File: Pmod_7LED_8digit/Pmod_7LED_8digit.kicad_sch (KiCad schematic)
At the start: 12 parts, among them IC1 TM1640, J1 Pmod_Header

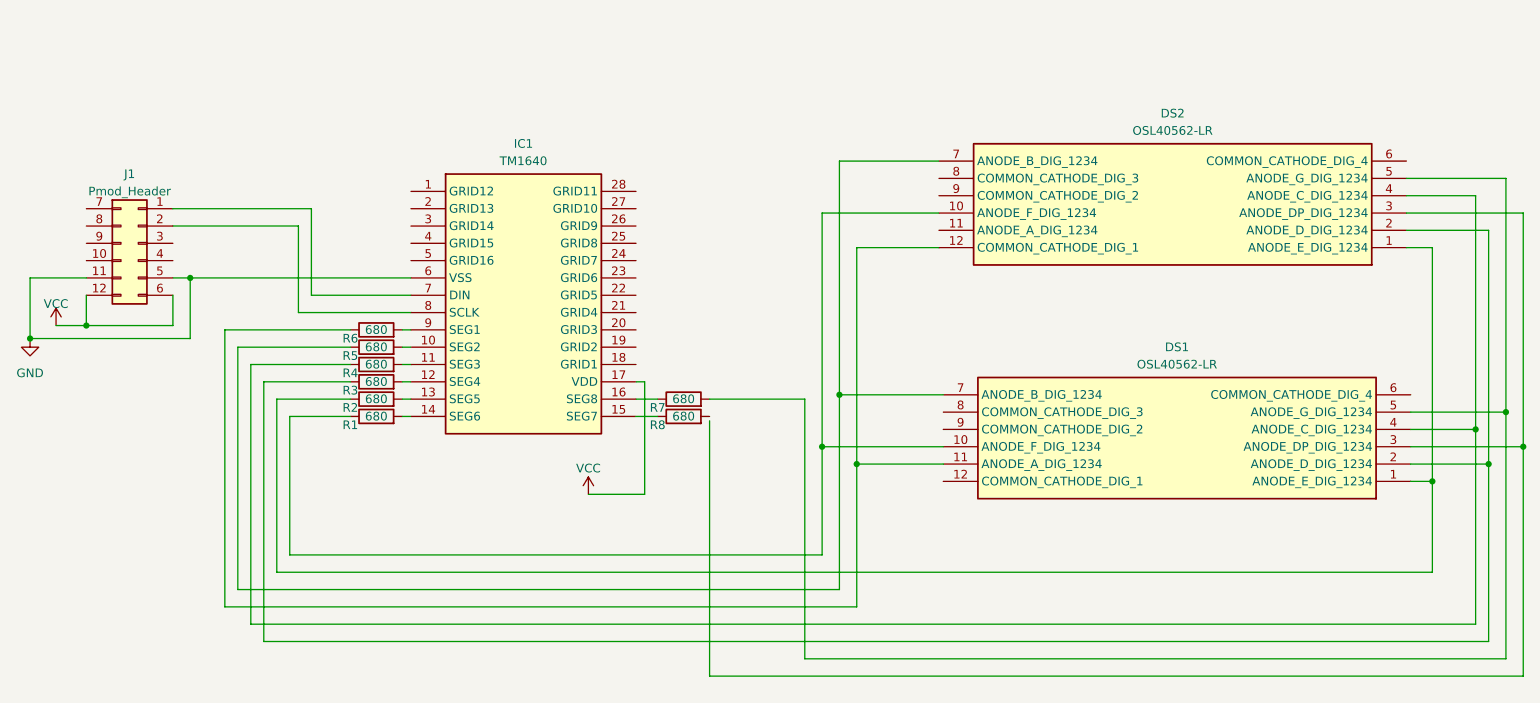
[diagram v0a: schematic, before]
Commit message: 0807
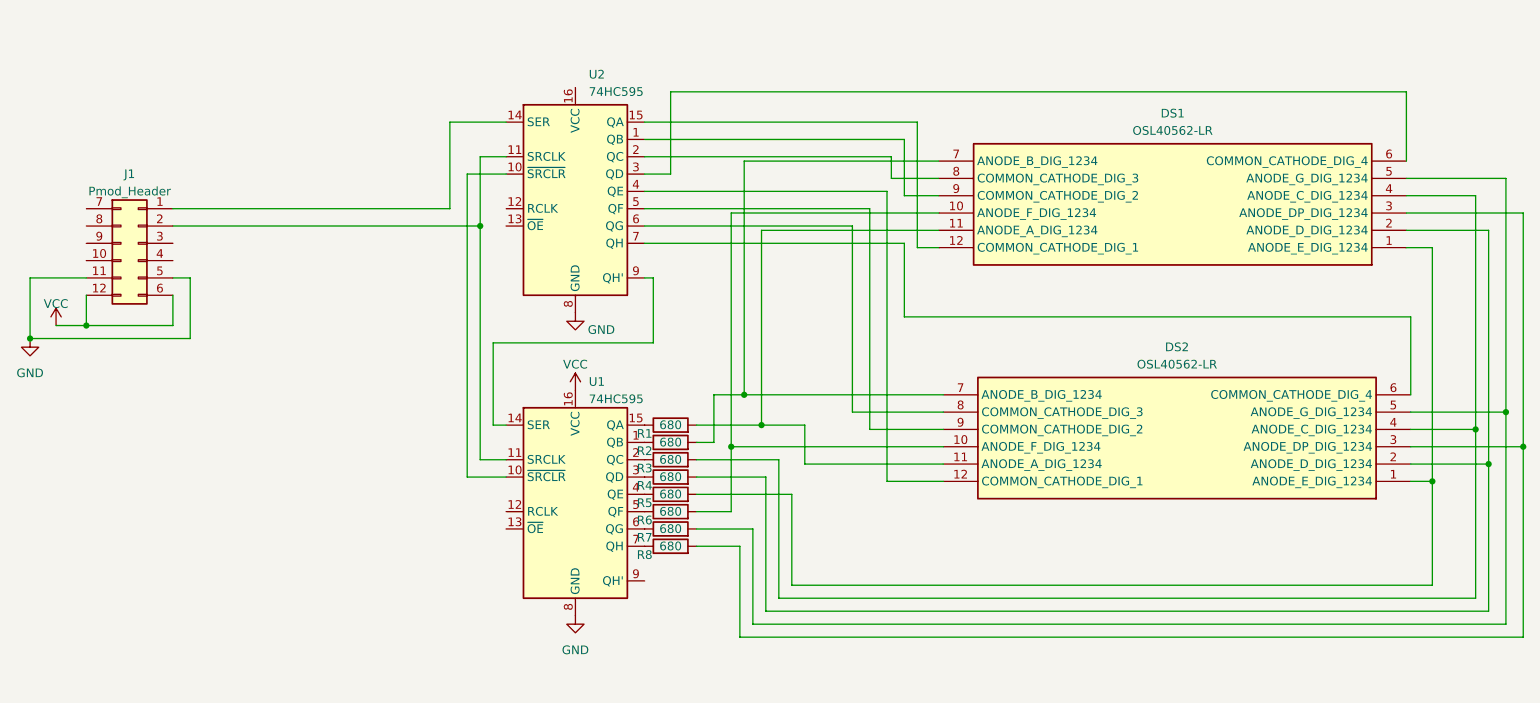
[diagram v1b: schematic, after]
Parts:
- removed IC1: TM1640, SOIC127P1020X269-28N, symbol SamacSys_Parts:TM1640
- added U1, U2: 74HC595, Package_SO:SOIC-16W_5.3x10.2mm_P1.27mm, symbol 74xx:74HC595
- renumbered DS2 to DS1, DS1 to DS2
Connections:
- net GND: now also U1.8 (GND), U2.8 (GND)
- net VCC: now also U1.16 (VCC)
- net at DS1.1 (ANODE_E_DIG_1234), DS2.1 (ANODE_E_DIG_1234): now also R5.2; no longer R2.1
- net at DS1.10 (ANODE_F_DIG_1234), DS2.10 (ANODE_F_DIG_1234): now also R6.2; no longer R1.1
- net at DS1.11 (ANODE_A_DIG_1234): now also DS2.11 (ANODE_A_DIG_1234), R1.2
- net at DS1.2 (ANODE_D_DIG_1234), DS2.2 (ANODE_D_DIG_1234): now also R4.2; no longer R3.1
- net at DS1.3 (ANODE_DP_DIG_1234), DS2.3 (ANODE_DP_DIG_1234): now also R8.2
- net at DS1.4 (ANODE_C_DIG_1234), DS2.4 (ANODE_C_DIG_1234): now also R3.2; no longer R4.1
- net at DS1.6 (COMMON_CATHODE_DIG_4): now also U2.3 (QD)
- net at DS1.7 (ANODE_B_DIG_1234), DS2.7 (ANODE_B_DIG_1234): now also R2.2; no longer R5.1
- net at DS1.8 (COMMON_CATHODE_DIG_3): now also U2.2 (QC)
- net at DS1.9 (COMMON_CATHODE_DIG_2): now also U2.1 (QB)
- net at R8.1: now also U1.7 (QH)
- net at R7.1: now also U1.6 (QG)
- net at J1.1 (Pin_1): now also U2.14 (SER)
- net at J1.2 (Pin_2): now also U1.11 (SRCLK), U2.11 (SRCLK)
- net at DS2.12 (COMMON_CATHODE_DIG_1): now also U2.4 (QE)
- net at DS2.6 (COMMON_CATHODE_DIG_4): now also U2.7 (QH)
- net at DS2.8 (COMMON_CATHODE_DIG_3): now also U2.6 (QG)
- net at DS2.9 (COMMON_CATHODE_DIG_2): now also U2.5 (QF)
- new net: DS1.12 (COMMON_CATHODE_DIG_1), U2.15 (QA)
- new net: R2.1, U1.1 (QB)
- new net: R1.1, U1.15 (QA)
- new net: U1.10 (~{SRCLR}), U2.10 (~{SRCLR})
- new net: U1.14 (SER), U2.9 (QH')
- new net: R3.1, U1.2 (QC)
- new net: R4.1, U1.3 (QD)
- new net: R5.1, U1.4 (QE)
- new net: R6.1, U1.5 (QF)
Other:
- moved on the sheet: R1, R2, R3, R4, R5, R6, R7, R8

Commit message: 0809
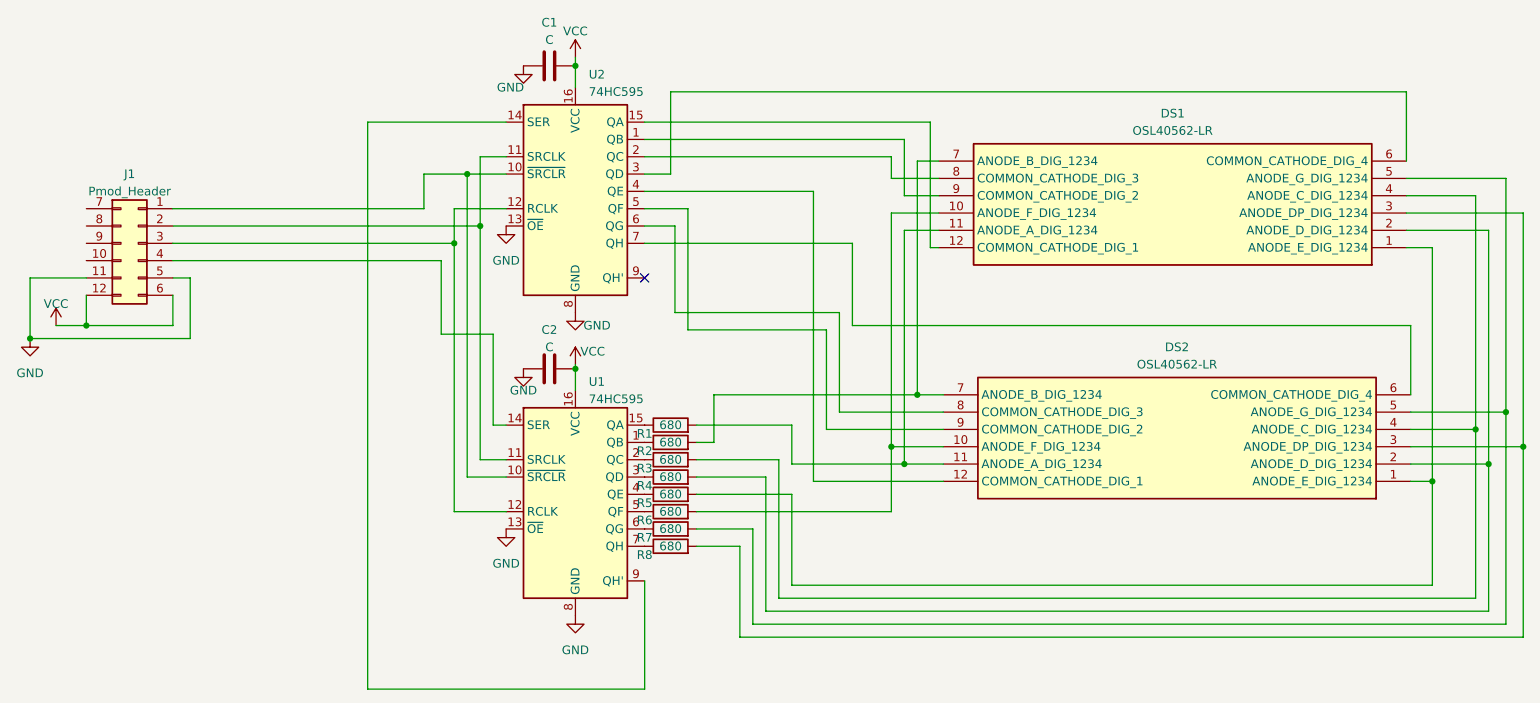
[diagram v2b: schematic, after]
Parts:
- added C1: C, Capacitor_SMD:C_0603_1608Metric_Pad1.08x0.95mm_HandSolder, symbol Device:C
- added C2: C, symbol Device:C
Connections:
- net GND: now also U1.13 (~{OE}), U2.13 (~{OE}), C1.2, C2.1
- net VCC: now also U2.16 (VCC), C1.1, C2.2
- net at U1.10 (~{SRCLR}), U2.10 (~{SRCLR}): now also J1.1 (Pin_1)
- net at U2.12 (RCLK): now also J1.3 (Pin_3), U1.12 (RCLK)
- net at U2.14 (SER): now also U1.9 (QH'); no longer J1.1 (Pin_1)
- net at U2.9 (QH'): no longer U1.14 (SER)
- net at J1.4 (Pin_4): now also U1.14 (SER)
- no-connect marks 0 -> 1

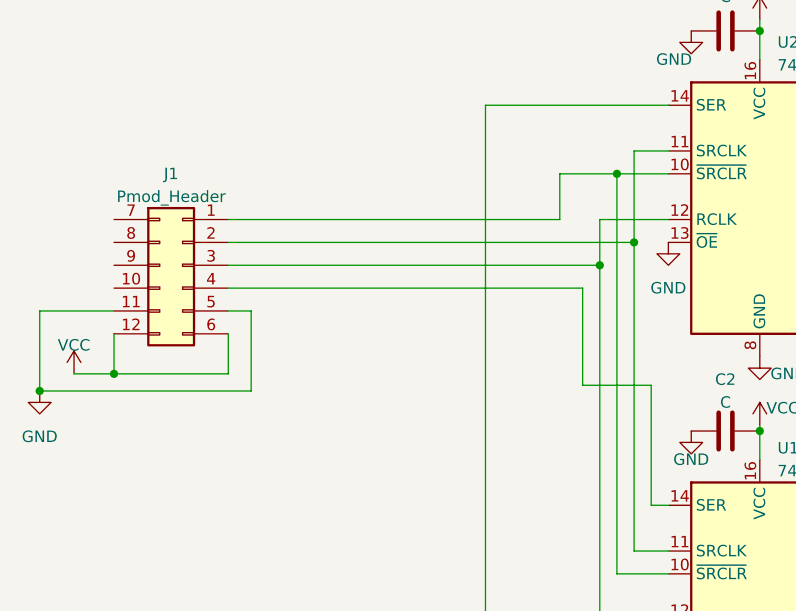
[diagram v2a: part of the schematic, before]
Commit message: 0811
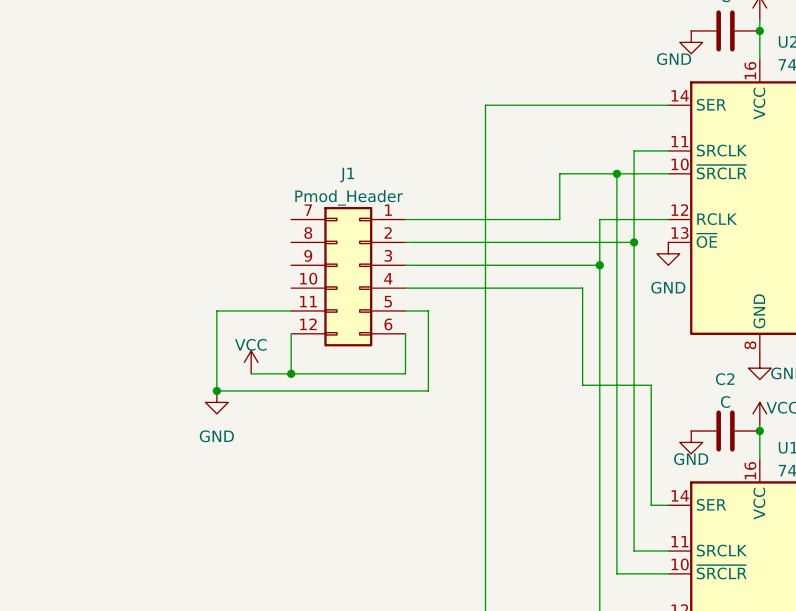
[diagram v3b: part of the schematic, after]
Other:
- moved on the sheet: J1
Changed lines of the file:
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@@
   (junction (at 111.76 67.945) (diameter 0) (color 0 0 0 0)
   )
-  (junction (at 31.75 107.95) (diameter 0) (color 0 0 0 0)
+  (junction (at 51.435 107.95) (diameter 0) (color 0 0 0 0)
   )
   (junction (at 93.98 93.98) (diameter 0) (color 0 0 0 0)
@@
   (junction (at 243.84 121.285) (diameter 0) (color 0 0 0 0)
   )
-  (junction (at 40.005 106.045) (diameter 0) (color 0 0 0 0)
+  (junction (at 59.69 106.045) (diameter 0) (color 0 0 0 0)
   )
   (junction (at 161.925 116.205) (diameter 0) (color 0 0 0 0)
@@
     (stroke (width 0) (type default))
   )
-  (wire (pts (xy 31.75 107.95) (xy 55.245 107.95))
+  (wire (pts (xy 51.435 107.95) (xy 74.93 107.95))
     (stroke (width 0) (type default))
   )
@@
     (stroke (width 0) (type default))
   )
-  (wire (pts (xy 55.245 99.06) (xy 52.705 99.06))
+  (wire (pts (xy 74.93 99.06) (xy 72.39 99.06))
     (stroke (width 0) (type default))
   )
@@
     (stroke (width 0) (type default))
   )
-  (wire (pts (xy 40.005 99.06) (xy 31.75 99.06))
+  (wire (pts (xy 59.69 99.06) (xy 51.435 99.06))
     (stroke (width 0) (type default))
   )
@@
     (stroke (width 0) (type default))
   )
-  (wire (pts (xy 52.705 88.9) (xy 89.535 88.9))
+  (wire (pts (xy 72.39 88.9) (xy 89.535 88.9))
     (stroke (width 0) (type default))
   )
@@
     (stroke (width 0) (type default))
   )
-  (wire (pts (xy 31.75 99.06) (xy 31.75 107.95))
+  (wire (pts (xy 51.435 99.06) (xy 51.435 107.95))
     (stroke (width 0) (type default))
   )
@@
     (stroke (width 0) (type default))
   )
-  (wire (pts (xy 52.705 101.6) (xy 52.705 106.045))
+  (wire (pts (xy 72.39 101.6) (xy 72.39 106.045))
     (stroke (width 0) (type default))
   )
@@
     (stroke (width 0) (type default))
   )
-  (wire (pts (xy 52.705 91.44) (xy 97.79 91.44))
+  (wire (pts (xy 72.39 91.44) (xy 97.79 91.44))
     (stroke (width 0) (type default))
   )
@@
     (stroke (width 0) (type default))
   )
-  (wire (pts (xy 92.075 96.52) (xy 52.705 96.52))
+  (wire (pts (xy 92.075 96.52) (xy 72.39 96.52))
     (stroke (width 0) (type default))
   )
@@
     (stroke (width 0) (type default))
   )
-  (wire (pts (xy 52.705 106.045) (xy 40.005 106.045))
+  (wire (pts (xy 72.39 106.045) (xy 59.69 106.045))
     (stroke (width 0) (type default))
   )
@@
     (stroke (width 0) (type default))
   )
-  (wire (pts (xy 35.56 106.045) (xy 40.005 106.045))
-    (stroke (width 0) (type default))
-  )
-  (wire (pts (xy 52.705 93.98) (xy 93.98 93.98))
+  (wire (pts (xy 55.245 106.045) (xy 59.69 106.045))
+    (stroke (width 0) (type default))
+  )
+  (wire (pts (xy 72.39 93.98) (xy 93.98 93.98))
     (stroke (width 0) (type default))
   )
@@
     (stroke (width 0) (type default))
   )
-  (wire (pts (xy 40.005 106.045) (xy 40.005 101.6))
+  (wire (pts (xy 59.69 106.045) (xy 59.69 101.6))
     (stroke (width 0) (type default))
   )
@@
     (stroke (width 0) (type default))
   )
-  (wire (pts (xy 55.245 99.06) (xy 55.245 107.95))
+  (wire (pts (xy 74.93 99.06) (xy 74.93 107.95))
     (stroke (width 0) (type default))
   )
@@
     )
   )
-  (symbol (lib_id "power:GND") (at 31.75 107.95 0) (unit 1)
+  (symbol (lib_id "power:GND") (at 51.435 107.95 0) (unit 1)
     (in_bom yes) (on_board yes) (dnp no) (fields_autoplaced)
-    (property "Reference" "#PWR03" (at 31.75 114.3 0)
-      (effects (font (size 1.27 1.27)) hide)
-    )
-    (property "Value" "GND" (at 31.75 113.03 0)
-      (effects (font (size 1.27 1.27)))
-    )
-    (property "Footprint" "" (at 31.75 107.95 0)
-      (effects (font (size 1.27 1.27)) hide)
-    )
-    (property "Datasheet" "" (at 31.75 107.95 0)
+    (property "Reference" "#PWR03" (at 51.435 114.3 0)
+      (effects (font (size 1.27 1.27)) hide)
+    )
+    (property "Value" "GND" (at 51.435 113.03 0)
+      (effects (font (size 1.27 1.27)))
+    )
+    (property "Footprint" "" (at 51.435 107.95 0)
+      (effects (font (size 1.27 1.27)) hide)
+    )
+    (property "Datasheet" "" (at 51.435 107.95 0)
       (effects (font (size 1.27 1.27)) hide)
     )
@@
     )
   )
-  (symbol (lib_id "power:VCC") (at 35.56 106.045 0) (unit 1)
+  (symbol (lib_id "power:VCC") (at 55.245 106.045 0) (unit 1)
     (in_bom yes) (on_board yes) (dnp no) (fields_autoplaced)
-    (property "Reference" "#PWR02" (at 35.56 109.855 0)
-      (effects (font (size 1.27 1.27)) hide)
-    )
-    (property "Value" "VCC" (at 35.56 102.87 0)
-      (effects (font (size 1.27 1.27)))
-    )
-    (property "Footprint" "" (at 35.56 106.045 0)
-      (effects (font (size 1.27 1.27)) hide)
-    )
-    (property "Datasheet" "" (at 35.56 106.045 0)
+    (property "Reference" "#PWR02" (at 55.245 109.855 0)
+      (effects (font (size 1.27 1.27)) hide)
+    )
+    (property "Value" "VCC" (at 55.245 102.87 0)
+      (effects (font (size 1.27 1.27)))
+    )
+    (property "Footprint" "" (at 55.245 106.045 0)
+      (effects (font (size 1.27 1.27)) hide)
+    )
+    (property "Datasheet" "" (at 55.245 106.045 0)
       (effects (font (size 1.27 1.27)) hide)
     )
@@
     )
   )
-  (symbol (lib_id "MyLibrary:Pmod_Header") (at 45.085 93.98 0) (unit 1)
+  (symbol (lib_id "MyLibrary:Pmod_Header") (at 64.77 93.98 0) (unit 1)
     (in_bom yes) (on_board yes) (dnp no) (fields_autoplaced)
-    (property "Reference" "J1" (at 46.355 83.82 0)
-      (effects (font (size 1.27 1.27)))
-    )
-    (property "Value" "Pmod_Header" (at 46.355 86.36 0)
-      (effects (font (size 1.27 1.27)))
-    )
-    (property "Footprint" "" (at 45.085 93.98 0)
-      (effects (font (size 1.27 1.27)) hide)
-    )
-    (property "Datasheet" "~" (at 45.085 93.98 0)
-      (effects (font (size 1.27 1.27)) hide)
-    )
+    (property "Reference" "J1" (at 66.04 83.82 0)
+      (effects (font (size 1.27 1.27)))
+    )
+    (property "Value" "Pmod_Header" (at 66.04 86.36 0)
+      (effects (font (size 1.27 1.27)))
+    )
+    (property "Footprint" "" (at 64.77 93.98 0)
+      (effects (font (size 1.27 1.27)) hide)
+    )
+    (property "Datasheet" "~" (at 64.77 93.98 0)
+      (effects (font (size 1.27 1.27)) hide)
+    )
